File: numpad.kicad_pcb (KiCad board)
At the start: 2 copper layers, 99.3 x 115.8 mm, 70 parts

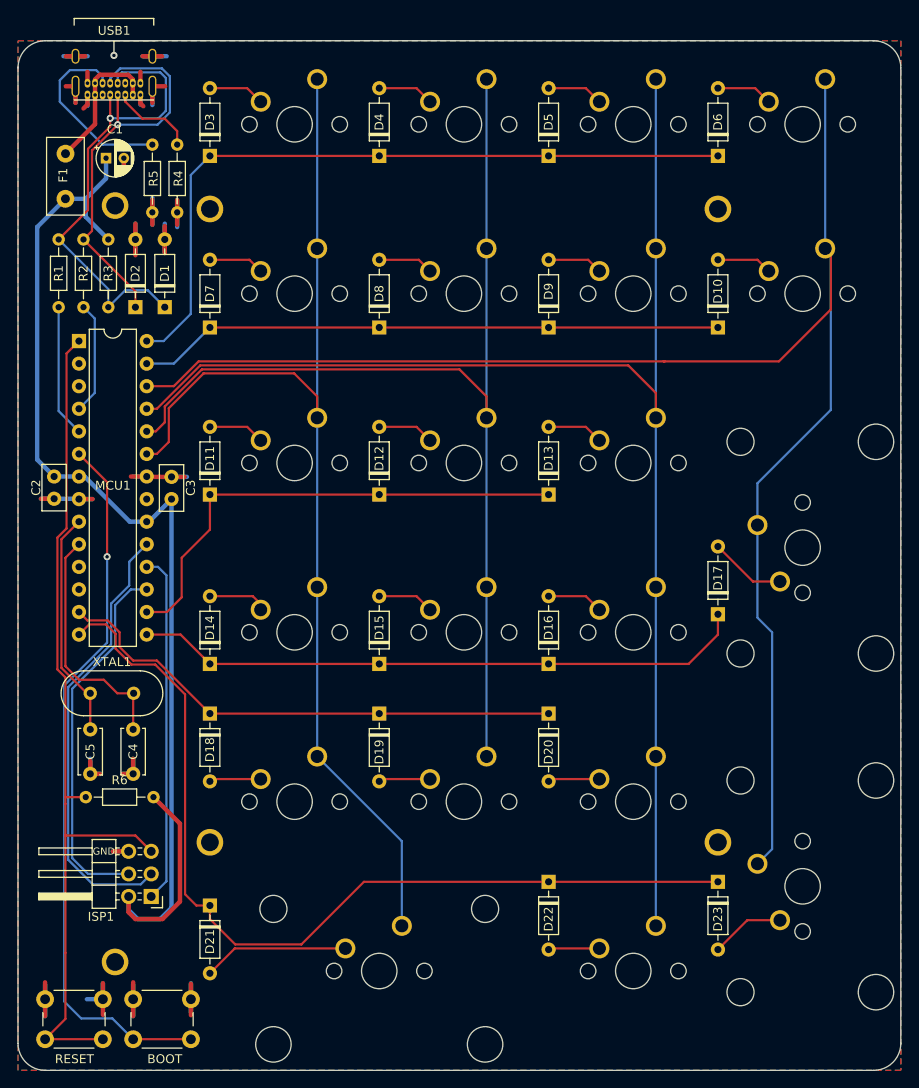
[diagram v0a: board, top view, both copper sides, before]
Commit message: update
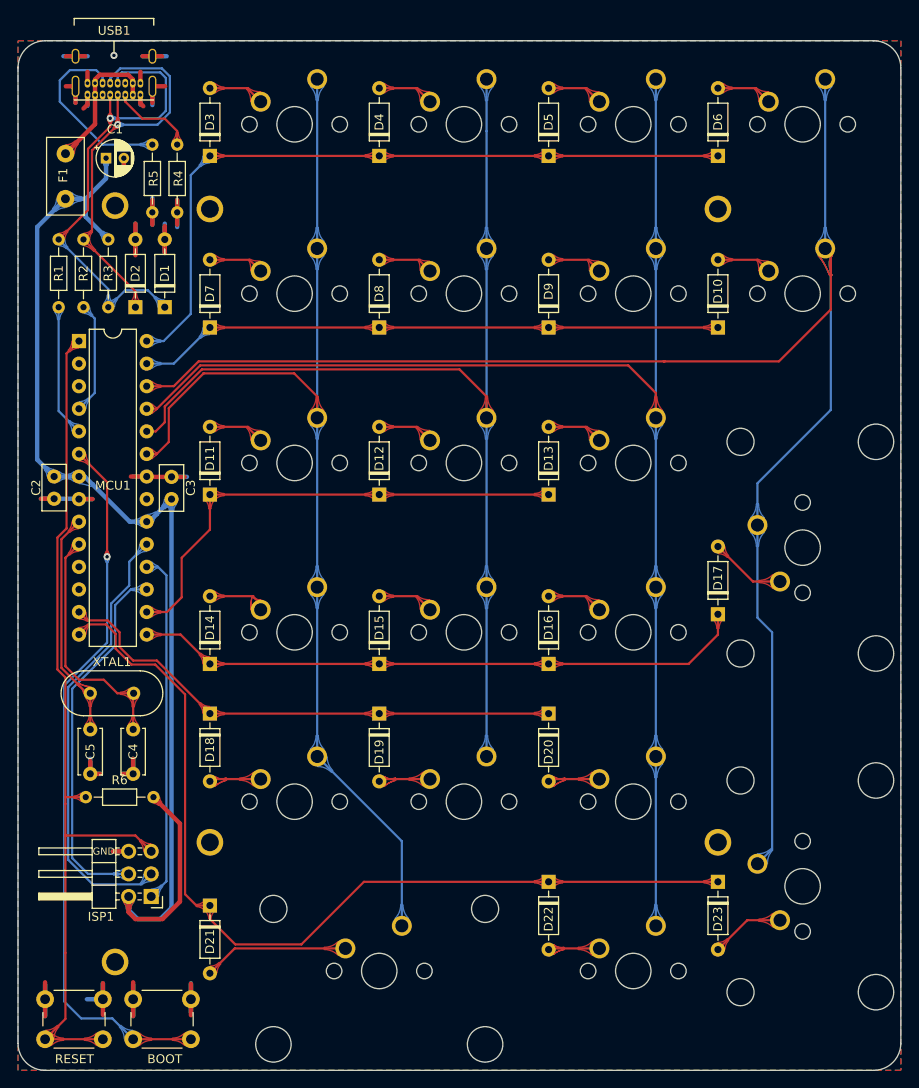
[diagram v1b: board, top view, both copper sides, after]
